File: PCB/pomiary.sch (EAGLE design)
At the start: 17 parts, among them IC2 LM358N

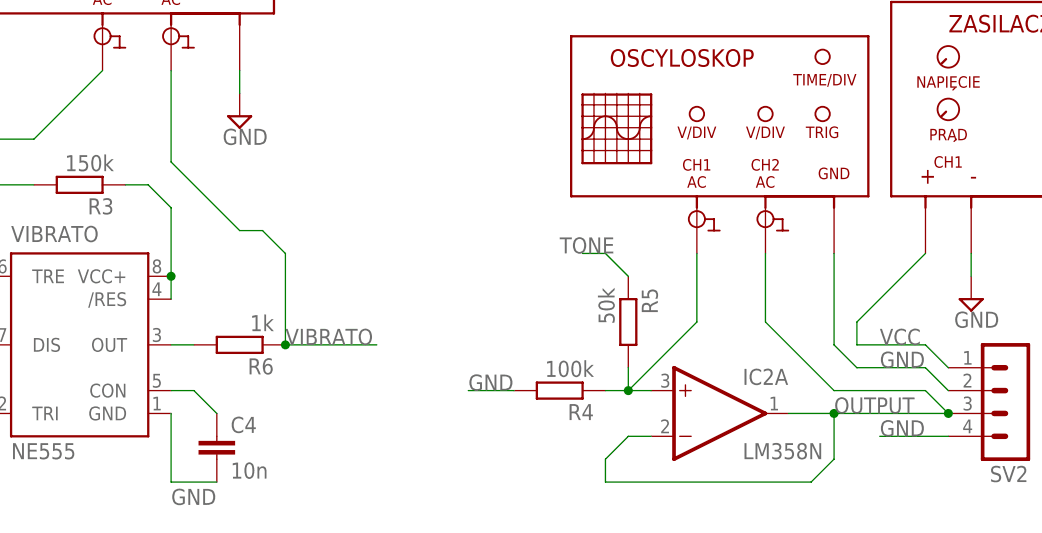
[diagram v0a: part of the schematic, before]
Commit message: almost finished
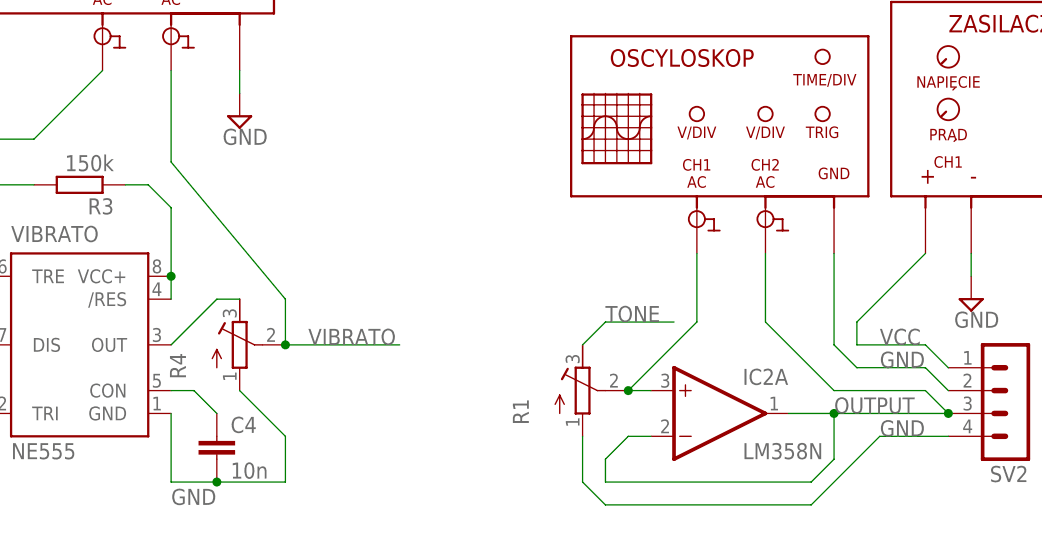
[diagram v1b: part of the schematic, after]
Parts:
- removed R5: 50k, resistor:R-EU_M1206
- removed R6: 1k, resistor:R-EU_M1206
- added R1: (no value), resistor:R-TRIMM5X
- R4: value 100k -> (none); device resistor:R-EU_M1206 -> resistor:R-TRIMM5X
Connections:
- removed net N$2: R6.2, VIBRATO.OUT
- new net N$4: R4.A, VIBRATO.OUT
- net GND: now also R1.E, R4.E; no longer R4.2
- net N$5: now also R1.S; no longer R4.1, R5.2
- net TONE: now also R1.A; no longer R5.1
- net VIBRATO: now also R4.S; no longer R6.1
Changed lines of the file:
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@@
 <part name="TONE" library="st-microelectronics" deviceset="NE555" device=""/>
 <part name="IC2" library="linear" deviceset="LM358" device="N"/>
-<part name="R4" library="resistor" deviceset="R-EU_" device="M1206" value="100k"/>
-<part name="R5" library="resistor" deviceset="R-EU_" device="M1206" value="50k"/>
 <part name="R2" library="resistor" deviceset="R-EU_" device="M1206" value="1k"/>
 <part name="C2" library="capacitor-wima" deviceset="C" device="2.5/5" value="100n"/>
@@
 <part name="C3" library="capacitor-wima" deviceset="C" device="2.5/5" value="1u"/>
 <part name="C4" library="capacitor-wima" deviceset="C" device="2.5/5" value="10n"/>
-<part name="R6" library="resistor" deviceset="R-EU_" device="M1206" value="1k"/>
 <part name="R7" library="resistor" deviceset="R-EU_" device="0204/7" value="10k"/>
 <part name="U$3" library="Przyrzady pomiarowe" deviceset="OSCYLOSKOP_AC_AC" device=""/>
@@
 <part name="U$4" library="Przyrzady pomiarowe" deviceset="OSCYLOSKOP_AC_AC" device=""/>
 <part name="SUPPLY4" library="supply2" deviceset="GND" device=""/>
+<part name="R1" library="resistor" deviceset="R-TRIMM" device="5X"/>
+<part name="R4" library="resistor" deviceset="R-TRIMM" device="5X"/>
 </parts>
 <sheets>
@@
 <instance part="TONE" gate="G$1" x="-271.78" y="121.92"/>
 <instance part="IC2" gate="A" x="-147.32" y="114.3"/>
-<instance part="R4" gate="G$1" x="-165.1" y="116.84" rot="R180"/>
-<instance part="R5" gate="G$1" x="-157.48" y="124.46" rot="R270"/>
 <instance part="R2" gate="G$1" x="-271.78" y="139.7" rot="R180"/>
 <instance part="C2" gate="G$1" x="-302.26" y="127"/>
@@
 <instance part="C3" gate="G$1" x="-243.84" y="127"/>
 <instance part="C4" gate="G$1" x="-203.2" y="111.76"/>
-<instance part="R6" gate="G$1" x="-200.66" y="121.92" rot="R180"/>
 <instance part="R7" gate="G$1" x="-236.22" y="139.7" rot="R180"/>
 <instance part="U$3" gate="G$1" x="-149.86" y="144.78"/>
@@
 <instance part="U$4" gate="G$1" x="-274.32" y="165.1"/>
 <instance part="SUPPLY4" gate="GND" x="-259.08" y="147.32"/>
+<instance part="R1" gate="G$1" x="-162.56" y="116.84"/>
+<instance part="R4" gate="G$1" x="-200.66" y="121.92"/>
 </instances>
 <busses>
@@
 <segment>
 <pinref part="IC2" gate="A" pin="+IN"/>
-<pinref part="R4" gate="G$1" pin="1"/>
 <wire x1="-154.94" y1="116.84" x2="-157.48" y2="116.84" width="0.1524" layer="91"/>
-<pinref part="R5" gate="G$1" pin="2"/>
-<wire x1="-157.48" y1="116.84" x2="-160.02" y2="116.84" width="0.1524" layer="91"/>
-<wire x1="-157.48" y1="119.38" x2="-157.48" y2="116.84" width="0.1524" layer="91"/>
-<junction x="-157.48" y="116.84"/>
 <pinref part="U$3" gate="G$1" pin="CH1"/>
 <wire x1="-149.86" y1="132.08" x2="-149.86" y2="124.46" width="0.1524" layer="91"/>
 <wire x1="-149.86" y1="124.46" x2="-157.48" y2="116.84" width="0.1524" layer="91"/>
+<pinref part="R1" gate="G$1" pin="S"/>
+<junction x="-157.48" y="116.84"/>
 </segment>
 </net>
 <net name="GND" class="0">
-<segment>
-<pinref part="R4" gate="G$1" pin="2"/>
-<label x="-175.26" y="116.84" size="1.778" layer="95"/>
-<wire x1="-170.18" y1="116.84" x2="-175.26" y2="116.84" width="0.1524" layer="91"/>
-</segment>
 <segment>
 <pinref part="SUPPLY1" gate="GND" pin="GND"/>
@@
 <wire x1="-208.28" y1="106.68" x2="-203.2" y2="106.68" width="0.1524" layer="91"/>
 <label x="-208.28" y="104.14" size="1.778" layer="95"/>
+<wire x1="-195.58" y1="106.68" x2="-203.2" y2="106.68" width="0.1524" layer="91"/>
+<junction x="-203.2" y="106.68"/>
+<pinref part="R4" gate="G$1" pin="E"/>
+<wire x1="-200.66" y1="116.84" x2="-195.58" y2="111.76" width="0.1524" layer="91"/>
+<wire x1="-195.58" y1="111.76" x2="-195.58" y2="106.68" width="0.1524" layer="91"/>
 </segment>
 <segment>
@@
 <wire x1="-121.92" y1="111.76" x2="-129.54" y2="111.76" width="0.1524" layer="91"/>
 <label x="-129.54" y="111.76" size="1.778" layer="95"/>
+<pinref part="R1" gate="G$1" pin="E"/>
+<wire x1="-162.56" y1="111.76" x2="-162.56" y2="106.68" width="0.1524" layer="91"/>
+<wire x1="-162.56" y1="106.68" x2="-160.02" y2="104.14" width="0.1524" layer="91"/>
+<wire x1="-160.02" y1="104.14" x2="-137.16" y2="104.14" width="0.1524" layer="91"/>
+<wire x1="-137.16" y1="104.14" x2="-129.54" y2="111.76" width="0.1524" layer="91"/>
 </segment>
 <segment>
@@
 </net>
 <net name="TONE" class="0">
-<segment>
-<pinref part="R5" gate="G$1" pin="1"/>
-<wire x1="-157.48" y1="129.54" x2="-160.02" y2="132.08" width="0.1524" layer="91"/>
-<wire x1="-160.02" y1="132.08" x2="-162.56" y2="132.08" width="0.1524" layer="91"/>
-<label x="-165.1" y="132.08" size="1.778" layer="95"/>
-</segment>
 <segment>
 <pinref part="TONE" gate="G$1" pin="OUT"/>
@@
 <wire x1="-266.7" y1="144.78" x2="-266.7" y2="152.4" width="0.1524" layer="91"/>
 </segment>
+<segment>
+<pinref part="R1" gate="G$1" pin="A"/>
+<wire x1="-162.56" y1="121.92" x2="-160.02" y2="124.46" width="0.1524" layer="91"/>
+<wire x1="-160.02" y1="124.46" x2="-152.4" y2="124.46" width="0.1524" layer="91"/>
+<label x="-160.02" y="124.46" size="1.778" layer="95"/>
+</segment>
 </net>
 <net name="VIBRATO" class="0">
@@
 </segment>
 <segment>
-<pinref part="R6" gate="G$1" pin="1"/>
-<wire x1="-195.58" y1="121.92" x2="-185.42" y2="121.92" width="0.1524" layer="91"/>
-<junction x="-195.58" y="121.92"/>
-<label x="-195.58" y="121.92" size="1.778" layer="95"/>
+<pinref part="R4" gate="G$1" pin="S"/>
+<wire x1="-195.58" y1="121.92" x2="-195.58" y2="127" width="0.1524" layer="91"/>
 <pinref part="U$2" gate="G$1" pin="CH2"/>
 <wire x1="-208.28" y1="152.4" x2="-208.28" y2="142.24" width="0.1524" layer="91"/>
-<wire x1="-208.28" y1="142.24" x2="-200.66" y2="134.62" width="0.1524" layer="91"/>
-<wire x1="-200.66" y1="134.62" x2="-198.12" y2="134.62" width="0.1524" layer="91"/>
-<wire x1="-198.12" y1="134.62" x2="-195.58" y2="132.08" width="0.1524" layer="91"/>
-<wire x1="-195.58" y1="132.08" x2="-195.58" y2="121.92" width="0.1524" layer="91"/>
+<wire x1="-195.58" y1="127" x2="-208.28" y2="142.24" width="0.1524" layer="91"/>
+<wire x1="-195.58" y1="121.92" x2="-182.88" y2="121.92" width="0.1524" layer="91"/>
+<junction x="-195.58" y="121.92"/>
+<label x="-193.04" y="121.92" size="1.778" layer="95"/>
 </segment>
 </net>
@@
 <pinref part="C4" gate="G$1" pin="1"/>
 <wire x1="-205.74" y1="116.84" x2="-203.2" y2="114.3" width="0.1524" layer="91"/>
-</segment>
-</net>
-<net name="N$2" class="0">
-<segment>
-<pinref part="VIBRATO" gate="G$1" pin="OUT"/>
-<pinref part="R6" gate="G$1" pin="2"/>
-<wire x1="-208.28" y1="121.92" x2="-205.74" y2="121.92" width="0.1524" layer="91"/>
 </segment>
 </net>
@@
 </segment>
 </net>
+<net name="N$4" class="0">
+<segment>
+<pinref part="VIBRATO" gate="G$1" pin="OUT"/>
+<wire x1="-208.28" y1="121.92" x2="-203.2" y2="127" width="0.1524" layer="91"/>
+<pinref part="R4" gate="G$1" pin="A"/>
+<wire x1="-203.2" y1="127" x2="-200.66" y2="127" width="0.1524" layer="91"/>
+</segment>
+</net>
